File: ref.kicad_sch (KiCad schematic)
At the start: 6 parts, among them Q1 Q_NPN_BCE, U4 ADR1000, U5 Opamp_Dual

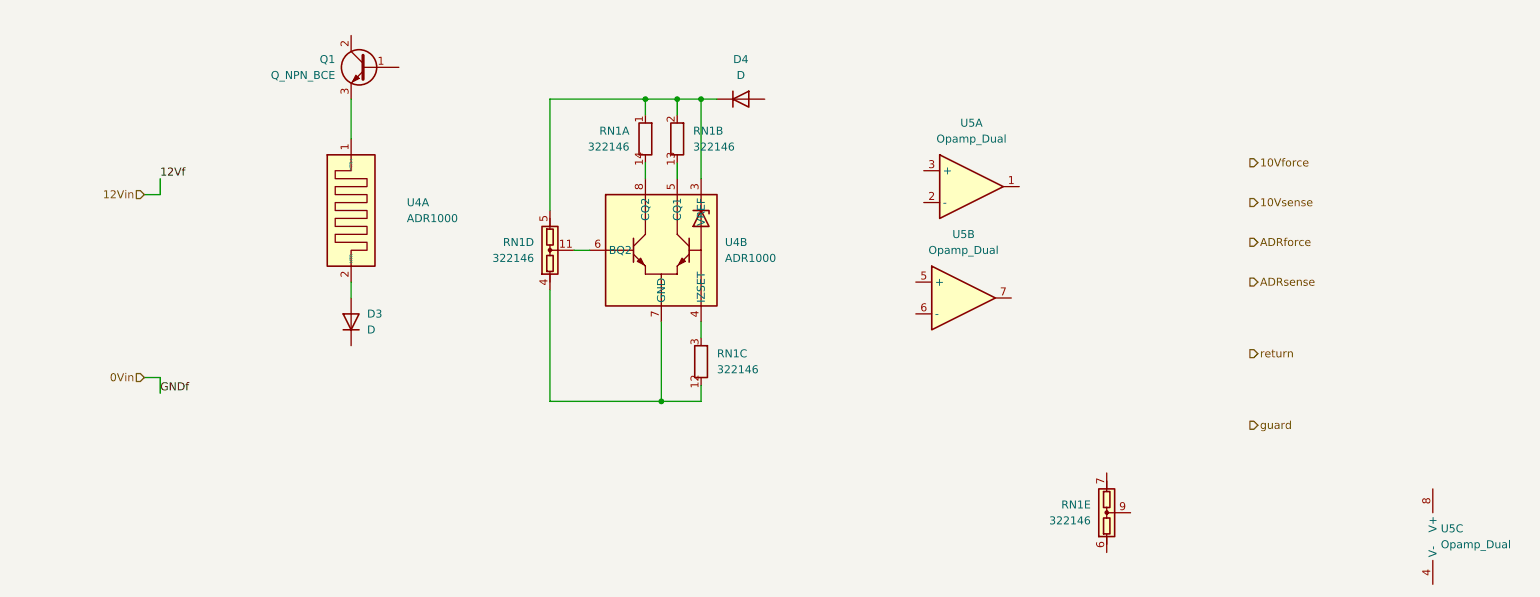
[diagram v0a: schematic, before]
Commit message: asdf
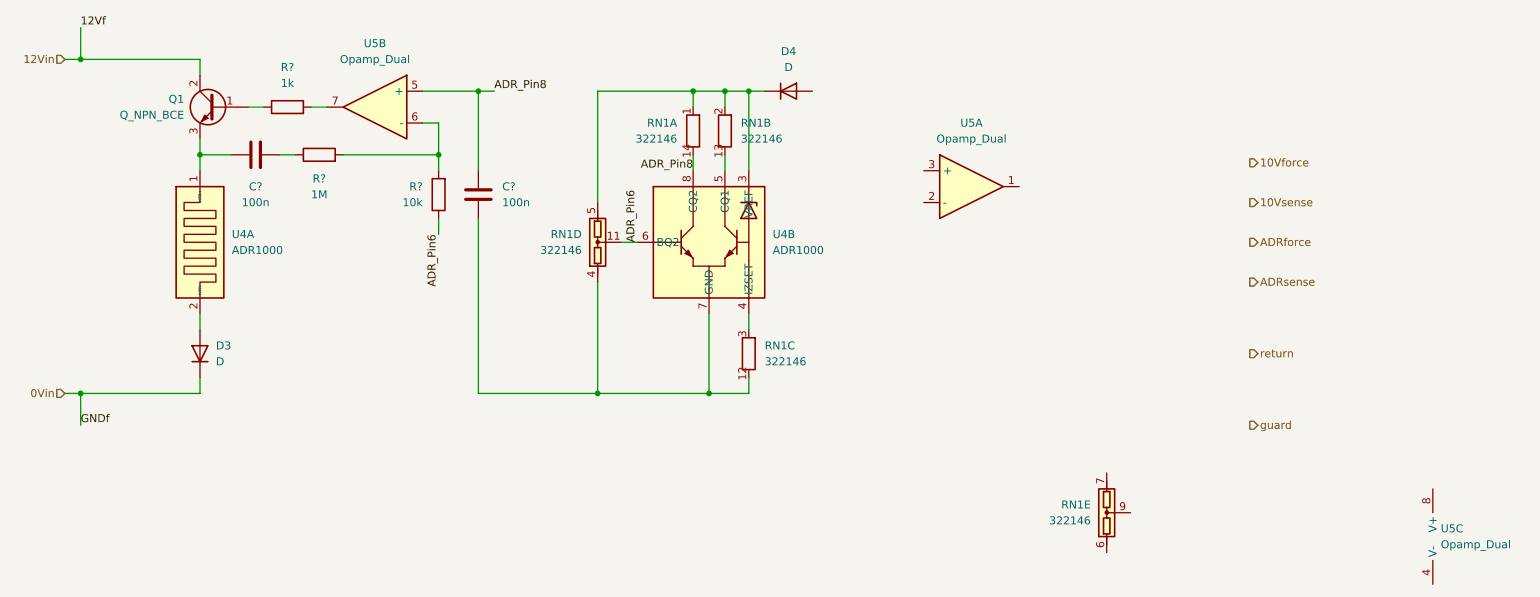
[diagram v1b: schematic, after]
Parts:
- added C? (x2): 100n, Capacitor_SMD:C_0805_2012Metric, symbol Device:C
- added R?: 1k, Resistor_SMD:R_0805_2012Metric, symbol Device:R
- added R?: 10k, Resistor_SMD:R_0805_2012Metric, symbol Device:R
- added R?: 1M, Resistor_SMD:R_0805_2012Metric, symbol Device:R
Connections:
- net 0Vin: now also D3.1 (K)
- net 12Vin: now also Q1.2 (C)
- net at Q1.3 (E), U4.1 (HTR+): now also C?.1
- net ADR_Pin6: now reaches RN1.11 (R4.2), U4.6 (BQ2)
- net ADR_Pin6: now also R?.1
- net at RN1.12 (R3.2), RN1.4 (R4.1), U4.7 (GND): now also C?.1
- net ADR_Pin8: now reaches RN1.14 (R1.2), U4.8 (CQ2)
- net ADR_Pin8: now also U5.5 (+), C?.2
- net at Q1.1 (B): now also R?.1
- net at U5.6 (-): now also R?.2, R?.2
- net at U5.7: now also R?.2
- new net: C?.2, R?.1
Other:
- moved on the sheet: D3, D4, Q1, RN1A, RN1B, RN1C, RN1D, U4A, U4B, U5B
